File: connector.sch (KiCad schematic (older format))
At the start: 1 part

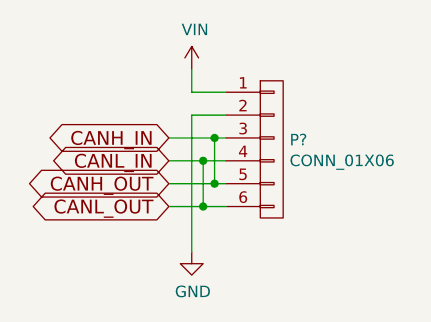
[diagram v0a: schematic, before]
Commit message: .
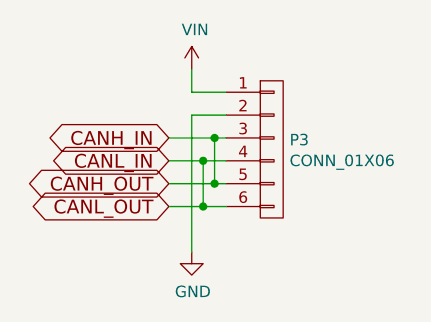
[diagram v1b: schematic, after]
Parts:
- P3: renamed from P?; footprint (none) -> Terminal_Blocks:TerminalBlock_WAGO-236_2Stift_RM5mm_6pol
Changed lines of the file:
@@
 $EndDescr
 $Comp
-L CONN_01X06 P?
+L CONN_01X06 P3
 U 1 1 57AF467D
 P 3400 4150
-F 0 "P?" H 3478 4191 50  0000 L CNN
+F 0 "P3" H 3478 4191 50  0000 L CNN
 F 1 "CONN_01X06" H 3478 4100 50  0000 L CNN
-F 2 "" H 3400 4150 50  0001 C CNN
+F 2 "Terminal_Blocks:TerminalBlock_WAGO-236_2Stift_RM5mm_6pol" H 3400 4150 50  0001 C CNN
 F 3 "" H 3400 4150 50  0000 C CNN
 	1    3400 4150
@@
 $EndComp
 $Comp
-L VIN #PWR?
+L VIN #PWR062
 U 1 1 57AF4ABC
 P 3050 3800
-F 0 "#PWR?" H 3050 3650 50  0001 C CNN
+F 0 "#PWR062" H 3050 3650 50  0001 C CNN
 F 1 "VIN" H 3065 3973 50  0000 C CNN
 F 2 "" H 3050 3800 60  0000 C CNN
@@
 	3050 3900 3050 3800
 $Comp
-L GND #PWR?
+L GND #PWR063
 U 1 1 57AF4B0E
 P 3050 4600
-F 0 "#PWR?" H 3050 4350 50  0001 C CNN
+F 0 "#PWR063" H 3050 4350 50  0001 C CNN
 F 1 "GND" H 3055 4427 50  0000 C CNN
 F 2 "" H 3050 4600 50  0000 C CNN
